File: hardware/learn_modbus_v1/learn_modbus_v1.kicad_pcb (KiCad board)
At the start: 2 copper layers, 11 parts, among them J1 SJ-43514-SMT, J3 RTU_CONN, U2 SeeeduinoXIAO, U3 THD301D485H

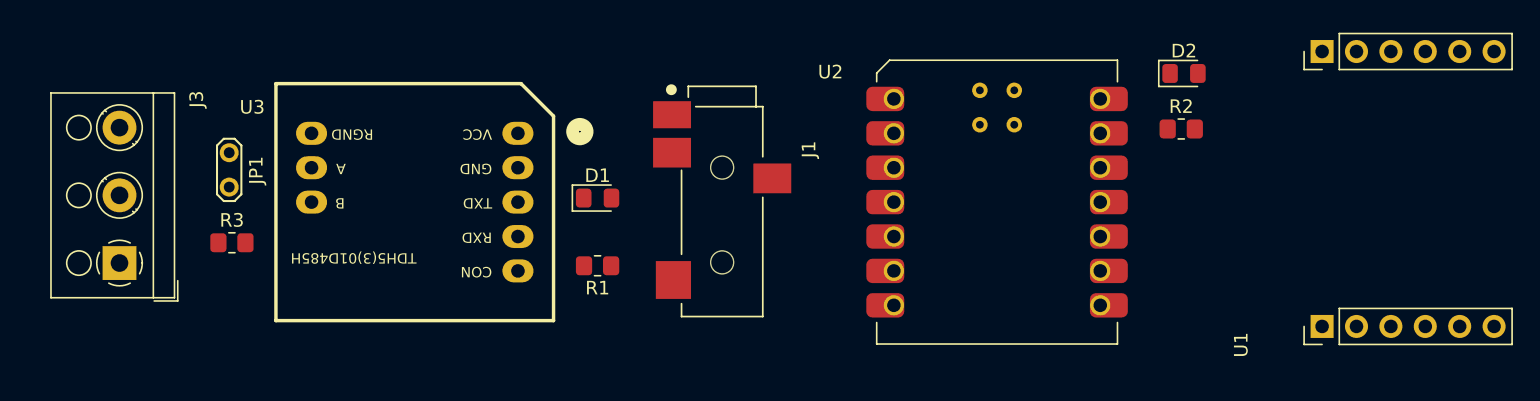
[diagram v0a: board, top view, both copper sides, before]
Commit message: hardware init
hardware init
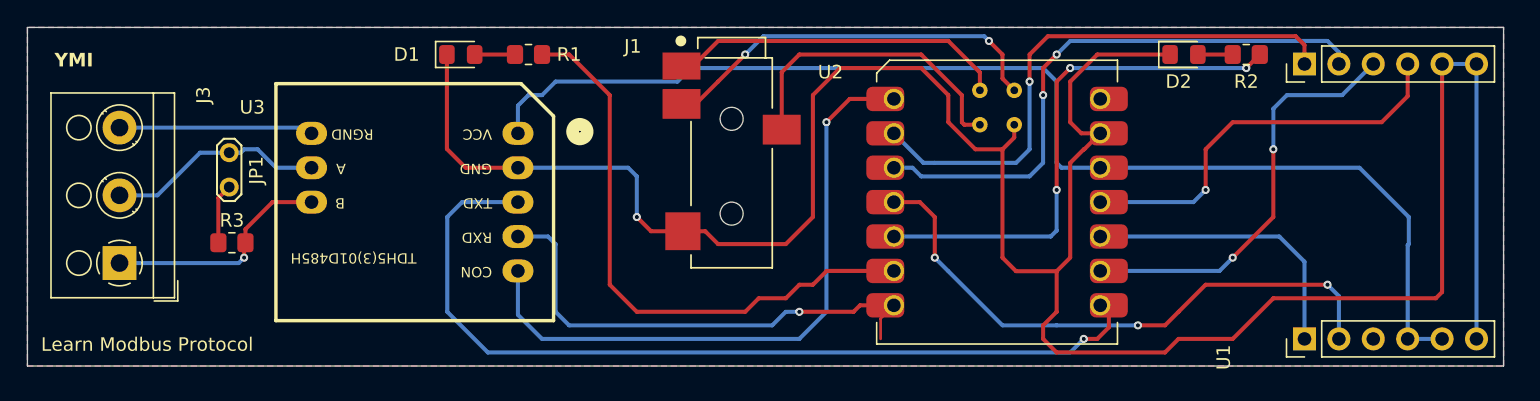
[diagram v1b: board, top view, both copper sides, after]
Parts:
- moved R1 16.4 mm to (115.0, 67.0)
- moved D1 14.6 mm to (110.0, 67.0)
- moved R2 7.30 mm to (168.0, 67.0), turned to 180 degrees
- moved J1 3.67 mm to (130.0, 75.0)
- moved U1 1.59 mm to (171.0, 89.4)
- moved D2 1.40 mm to (163.4, 67.0)
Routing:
- net GND: track 0.00 -> 183.9 mm, vias 0 -> 1
- net PWR_3V3: track 0.00 -> 88.6 mm
- net RTU_TX: track 0.00 -> 65.2 mm, vias 0 -> 1
- net RTU_EN: track 0.00 -> 46.6 mm, vias 0 -> 1
- net ETH_RST: track 0.00 -> 43.1 mm, vias 0 -> 3
- net RTU_LED: track 0.00 -> 42.7 mm
- net ETH_CS: track 0.00 -> 42.6 mm, vias 0 -> 2
- net ETH_INT: track 0.00 -> 40.9 mm, vias 0 -> 1
- net ETH_LED: track 0.00 -> 39.0 mm, vias 0 -> 3
- net RTU_RX: track 0.00 -> 36.3 mm, vias 0 -> 1
- net ETH_SCLK: track 0.00 -> 31.2 mm, vias 0 -> 2
- net PRG_SWCLK: track 0.00 -> 30.3 mm, vias 0 -> 2
- net ETH_MOSI: track 0.00 -> 30.1 mm, vias 0 -> 1
- net PRG_SWDIO: track 0.00 -> 25.1 mm
- net PRG_RST: track 0.00 -> 22.7 mm
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- added copper zone on B.Cu, net GND
- added copper zone on F.Cu, net GND
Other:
- board outline added: 109 x 25 mm
- board text added: "AUD-1 -- SWDIO AUD-2 -- GND AUD-3 -- RST AUD-4 -- SWCLK"
- board text added: "D0 -- RTU Con D5 -- RTU Led"
- board text added: "D1 -- TCP INT D2 -- TCP CS D3 -- TCP RST D5 -- TCP LED MISO -- TCP MISO MOSI -- TCP MOSI SCLK -- TCP SCLK"
- board text added: "Learn Modbus Protocol"
- board text added: "Modbus RTU Modbus ASCII Modbus TCPIP"
- board text added: "TX -- RTU Rx RX -- RTU Tx"
- board text added: "YMI"
